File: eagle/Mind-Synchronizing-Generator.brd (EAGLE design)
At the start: 160 x 100 mm, 30 parts, among them IC1 555_ALT2, IC2 555_ALT2, IC3 555_ALT2

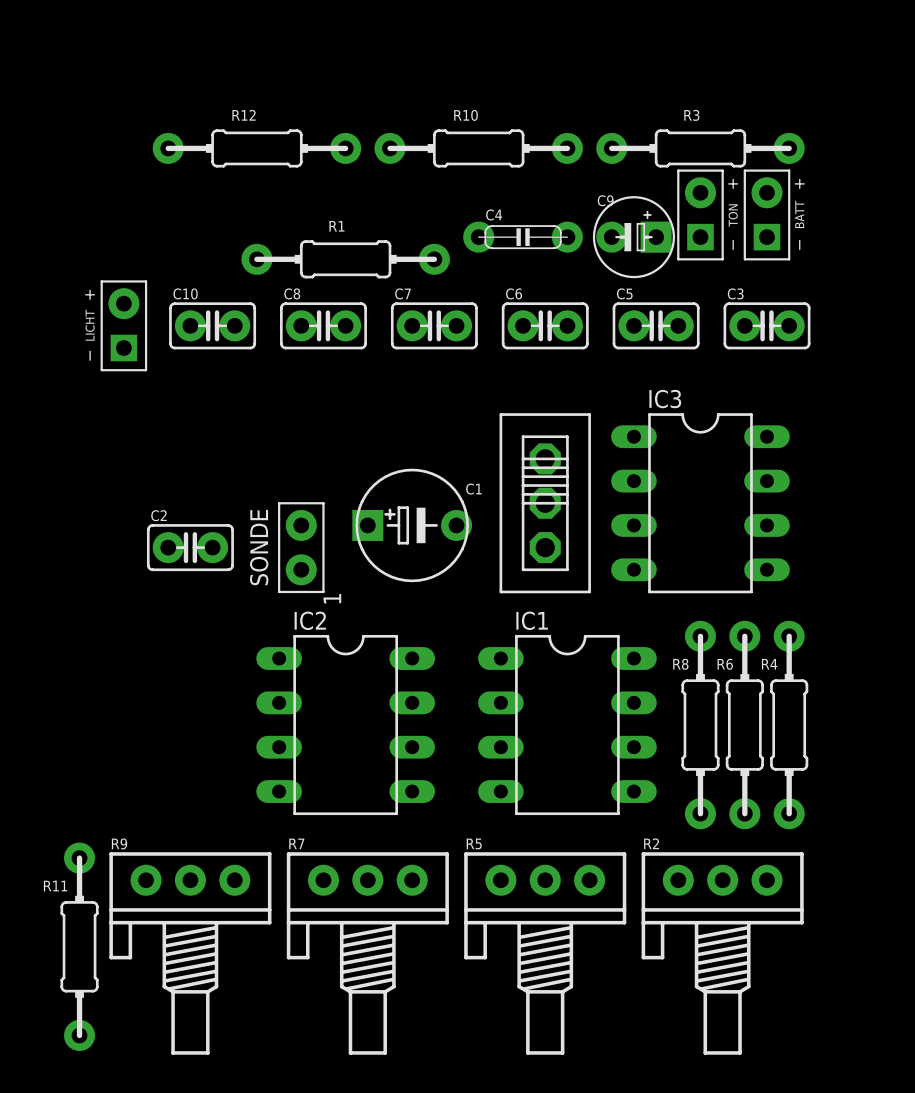
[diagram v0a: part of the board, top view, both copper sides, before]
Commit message: ...
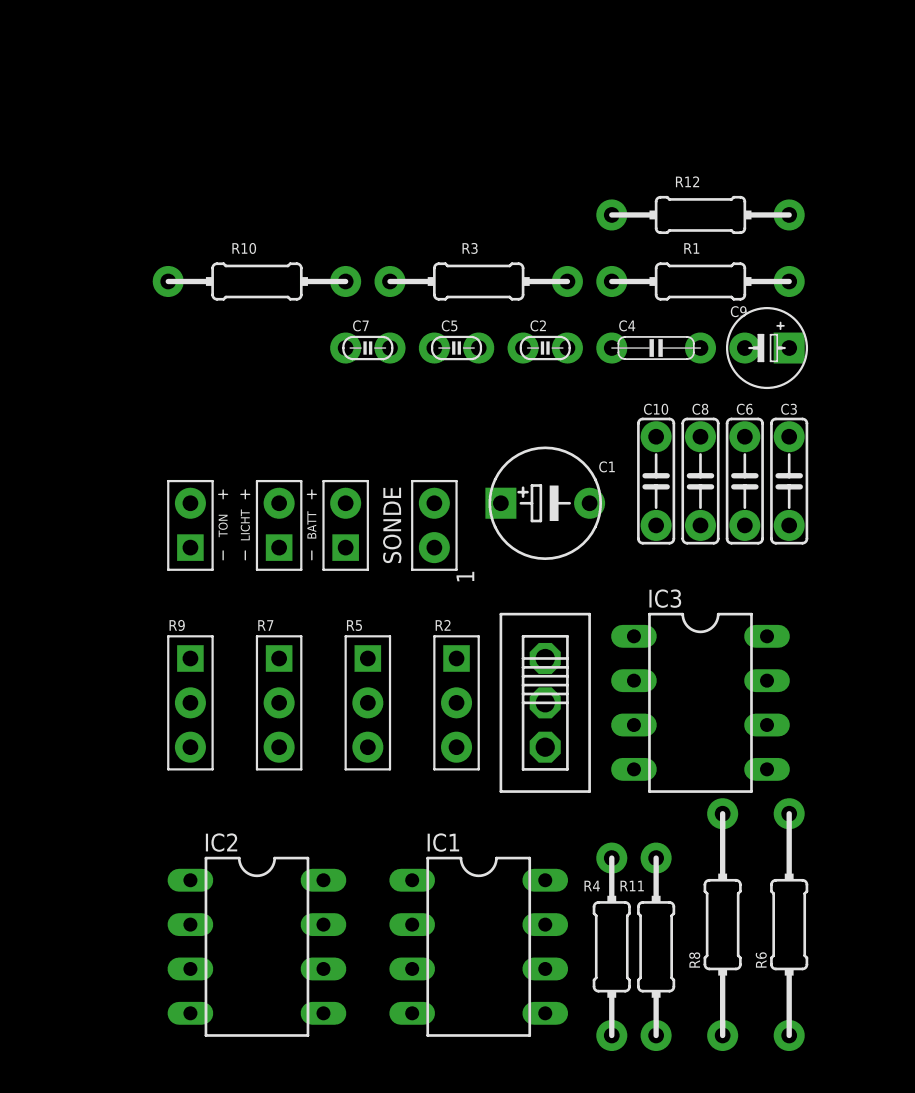
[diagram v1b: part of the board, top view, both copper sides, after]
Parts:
- BATT: value SPAD+-+- -> SPAD+--+; device pad:SPAD+- -> pad:SPAD-+
- C10, C3, C6, C8: device c:C025-025X050 -> c:C050-025X060
- C2, C5, C7: device c:C025-025X050 -> c:C025-015X024
- R2, R5, R7, R9: device r:POT -> r:CONN-3P
- R6, R8: device r:0204/10-V -> r:0204/12-V
- moved TON 34.2 mm to (-48.3, 30.5)
- moved R11 33.0 mm to (-21.6, 6.35)
- moved BATT 30.0 mm to (-39.4, 30.5)
- moved C10 26.9 mm to (-21.6, 33.0)
- moved R12 25.7 mm to (-19.1, 48.3)
- moved C8 23.3 mm to (-19.1, 33.0)
- moved C2 23.3 mm to (-27.9, 40.6)
- moved R1 20.4 mm to (-19.1, 44.5)
- moved R2 18.3 mm to (-33.0, 20.3)
- moved R4 16.3 mm to (-24.1, 6.35)
- moved R10 14.8 mm to (-44.5, 44.5)
- moved R3 14.8 mm to (-31.8, 44.5)
- moved LICHT 14.5 mm to (-43.2, 30.5)
- moved C6 14.5 mm to (-16.5, 33.0)
- moved R5 14.4 mm to (-38.1, 20.3)
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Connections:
- removed net N$10: IC2.3, IC3.4, R7.E, R8.2
- removed net N$14: C9.+, IC3.3, R9.A
- removed net N$4: C4.1, IC1.3, R1.1, R2.A
- new net Q1: C4.1, IC1.3, R1.1, R2.1, SONDE.1
- new net Q2: IC2.3, IC3.4, R7.3, R8.2
- new net Q3: C9.+, IC3.3, R9.1
- net N$11: now also R7.1, R7.2; no longer R7.A, R7.S
- net N$13: now also R9.2, R9.3; no longer R9.E, R9.S
- net N$3: now also R2.2, R2.3; no longer R2.E, R2.S
- net N$6: now also SONDE.2; no longer SONDE.1
- net N$8: now also R5.1; no longer R5.A
- net VCC: now also R5.2, R5.3; no longer R5.E, R5.S
